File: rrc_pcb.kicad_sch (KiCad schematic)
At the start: 13 parts, among them J1 Voltage Regulator Input, J2 Conn_01x03_Male, U1 ADXL357Z, U2 Teensy3.6-teensy, U3 BN220-GPS, U4 MS5611, U5 logo

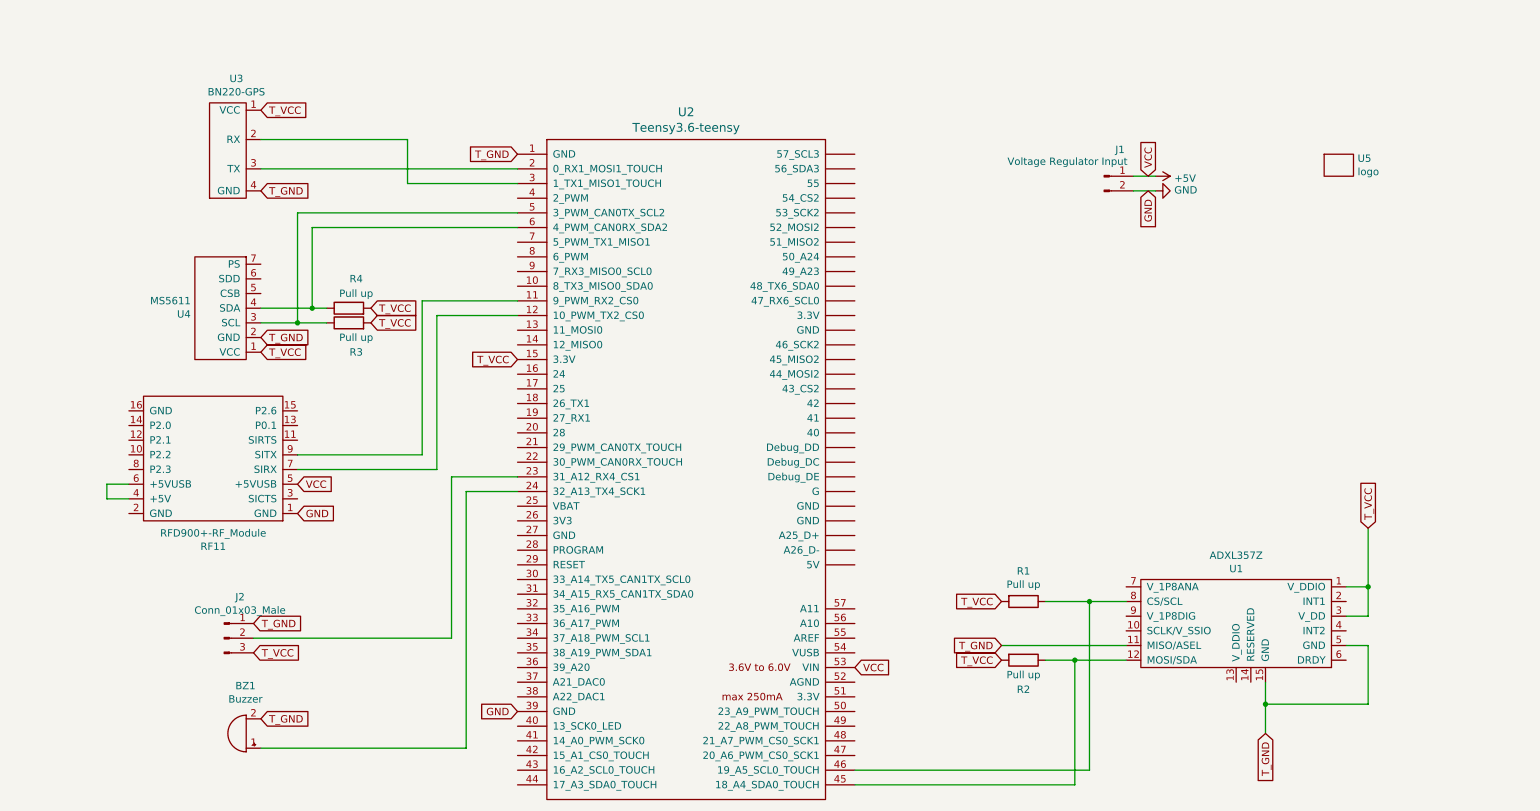
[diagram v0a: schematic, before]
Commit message: updated .sch
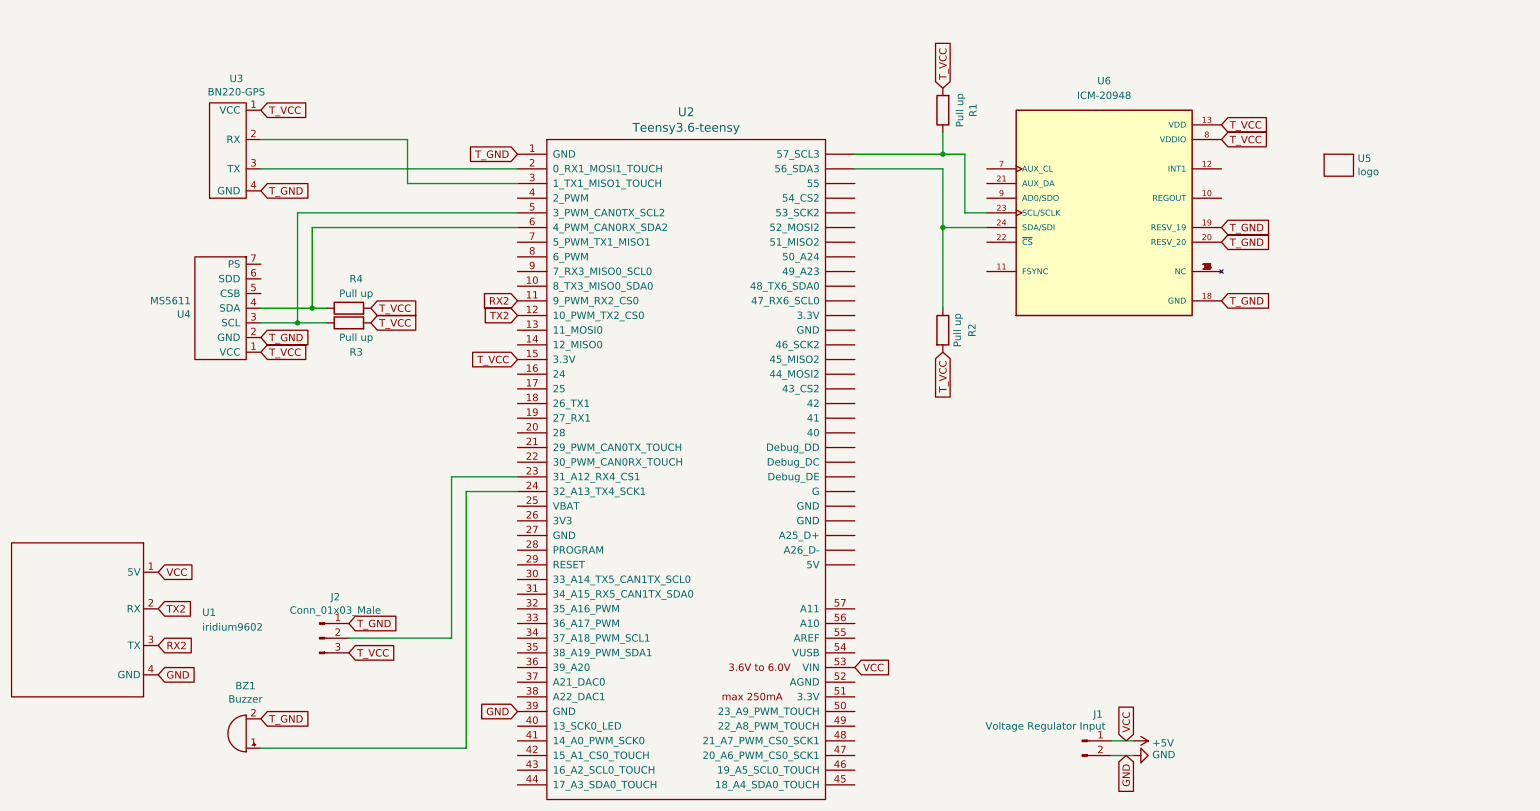
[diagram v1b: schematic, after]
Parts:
- removed RF11: RFD900+-RF_Module, rfd900+:RFD900+, symbol parts:RFD900+-RF_Module
- removed U1: ADXL357Z, adxl357z:ADXL357, symbol parts:ADXL357Z
- added U1: iridium9602, symbol parts:iridium9602
- added U6: ICM-20948, QFN40P300X300X105-24N, symbol parts:ICM-20948
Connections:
- net +5V: now also U1.1 (5V)
- net GND: now also U1.4 (GND)
- net T_GND: now also U6.18 (GND), U6.19 (RESV_19), U6.20 (RESV_20)
- net T_VCC: now also U6.13 (VDD), U6.8 (VDDIO)
- net RX2: now reaches U2.11 (9_PWM_RX2_CS0)
- net RX2: now also U1.3 (TX)
- net TX2: now reaches U2.12 (10_PWM_TX2_CS0)
- net TX2: now also U1.2 (RX)
- net at U2.45 (18_A4_SDA0_TOUCH): no longer R2.1
- net at U2.46 (19_A5_SCL0_TOUCH): no longer R1.1
- net at U2.~ (GND): now also R2.1, U6.24 (SDA/SDI)
- new net: R1.1, U2.~ (GND), U6.23 (SCL/SCLK)
- new net: U6.1 (NC), U6.14 (NC), U6.15 (NC), U6.16 (NC), U6.17 (NC), U6.2 (NC), U6.3 (NC), U6.4 (NC), U6.5 (NC), U6.6 (NC)
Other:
- moved on the sheet: J1, J2, R1, R2

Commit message: update 2
updated .sch added teensy4.1 , and updated footprints. Still in debugging stage
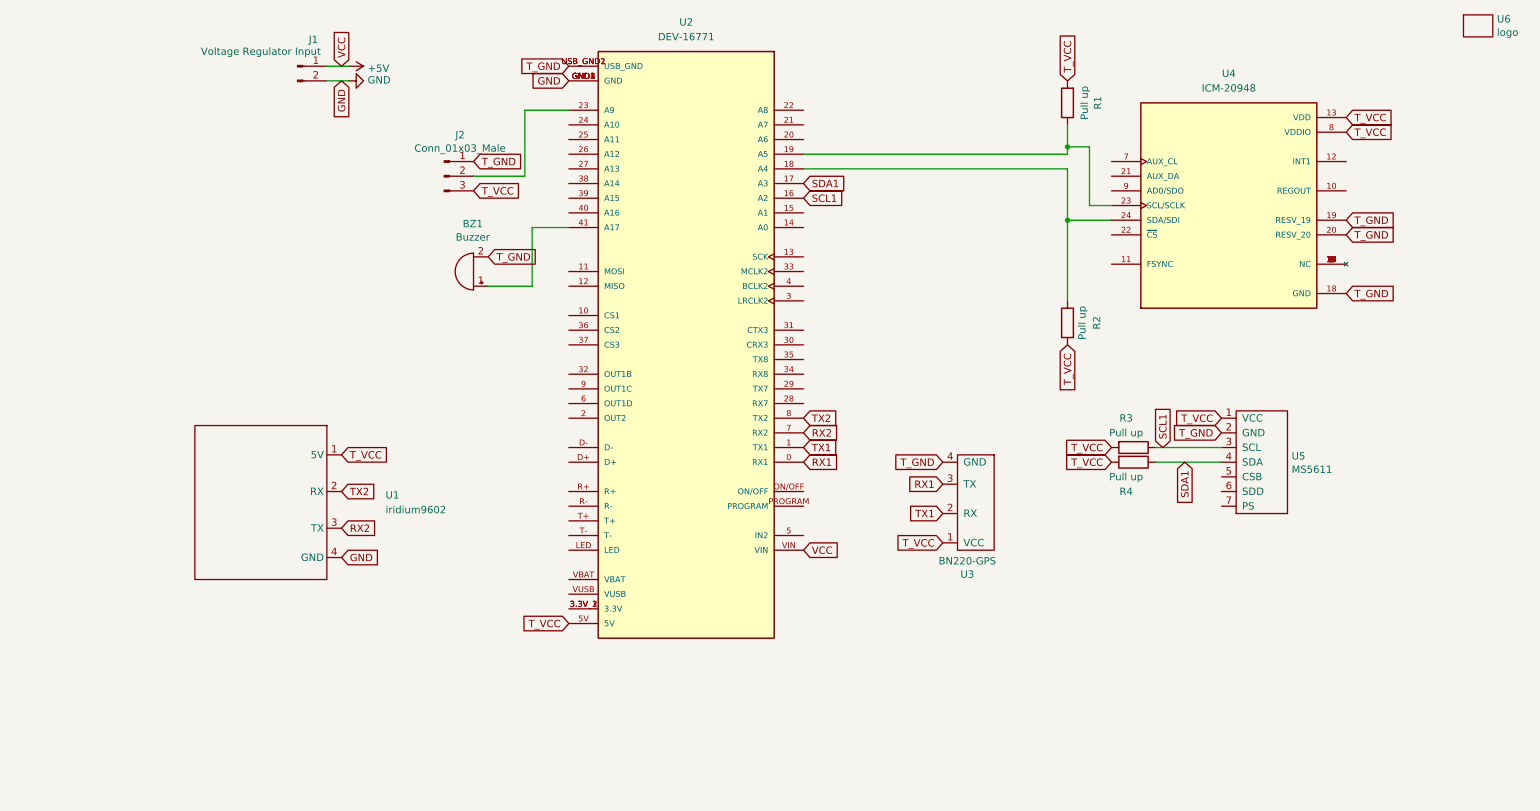
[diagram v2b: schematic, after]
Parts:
- removed U2: Teensy3.6-teensy, teensy:Teensy35_36, symbol parts:Teensy3.6-teensy
- added U2: DEV-16771, teensy:Teensy41, symbol parts:DEV-16771
- U1: footprint (none) -> Connector_PinHeader_2.54mm:PinHeader_1x04_P2.54mm_Horizontal
- U4: renamed from U6; footprint QFN40P300X300X105-24N -> Connector_PinHeader_2.54mm:PinHeader_2x10_P2.54mm_Vertical
- renumbered U4 to U5, U5 to U6
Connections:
- net +5V: now also U2.VIN; no longer U1.1 (5V)
- net GND: now also U2.GND1 (GND), U2.GND2 (GND), U2.GND3 (GND), U2.GND4 (GND), U2.GND5 (GND)
- net RX2: now also U2.7 (RX2)
- net TX2: now also U2.8 (TX2)
- net T_GND: now also U2.USB_GND1 (USB_GND), U2.USB_GND2 (USB_GND)
- net T_VCC: now also U1.1 (5V), U2.5V
- net RX1: now reaches U3.3 (TX)
- net RX1: now also U2.0 (RX1)
- net at J2.2 (Pin_2): now also U2.23 (A9)
- net at BZ1.1 (-): now also U2.41 (A17)
- net TX1: now reaches U3.2 (RX)
- net TX1: now also U2.1 (TX1)
- net SCL1: now reaches R3.1, U5.3 (SCL)
- net SCL1: now also U2.16 (A2)
- net SDA1: now reaches R4.1, U5.4 (SDA)
- net SDA1: now also U2.17 (A3)
- net at R1.1, U4.23 (SCL/SCLK): now also U2.19 (A5)
- net at R2.1, U4.24 (SDA/SDI): now also U2.18 (A4)
- new net: U2.3.3V_1 (3.3V), U2.3.3V_2 (3.3V), U2.3.3V_3 (3.3V)
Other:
- moved on the sheet: BZ1, J1, J2, R1, R2, R3, R4, U1, U3, U4, U5, U6
